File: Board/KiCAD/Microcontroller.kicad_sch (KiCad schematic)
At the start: 29 parts, among them J2 Conn_ARM_SWD_TagConnect_TC2030, J4 Conn_01x03, SW2 SW_Push, U5 LMR50410, U9 STM32F103C8T6, Y1 Crystal_GND24_Small, Y4 CM8V-T1A-32.768KHZ-12.5PF-20P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

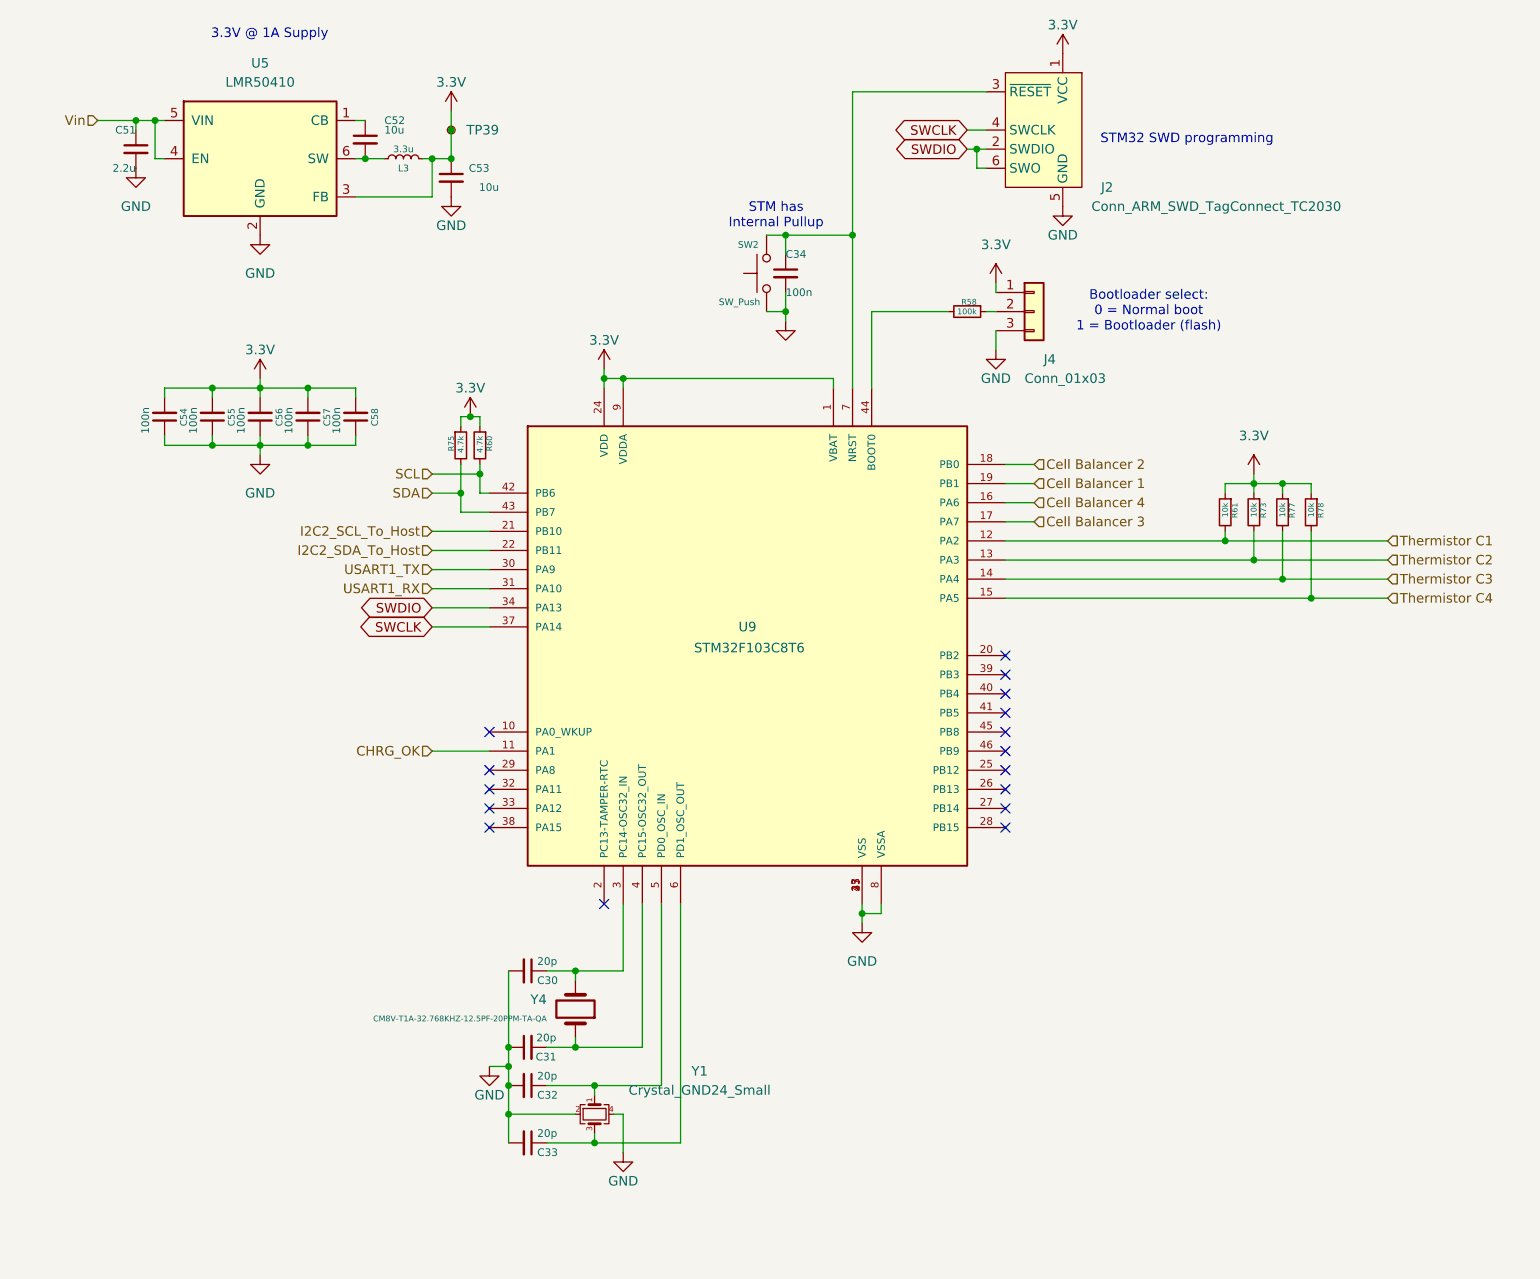
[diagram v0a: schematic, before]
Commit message: BOM Complete Need a Once Over Check
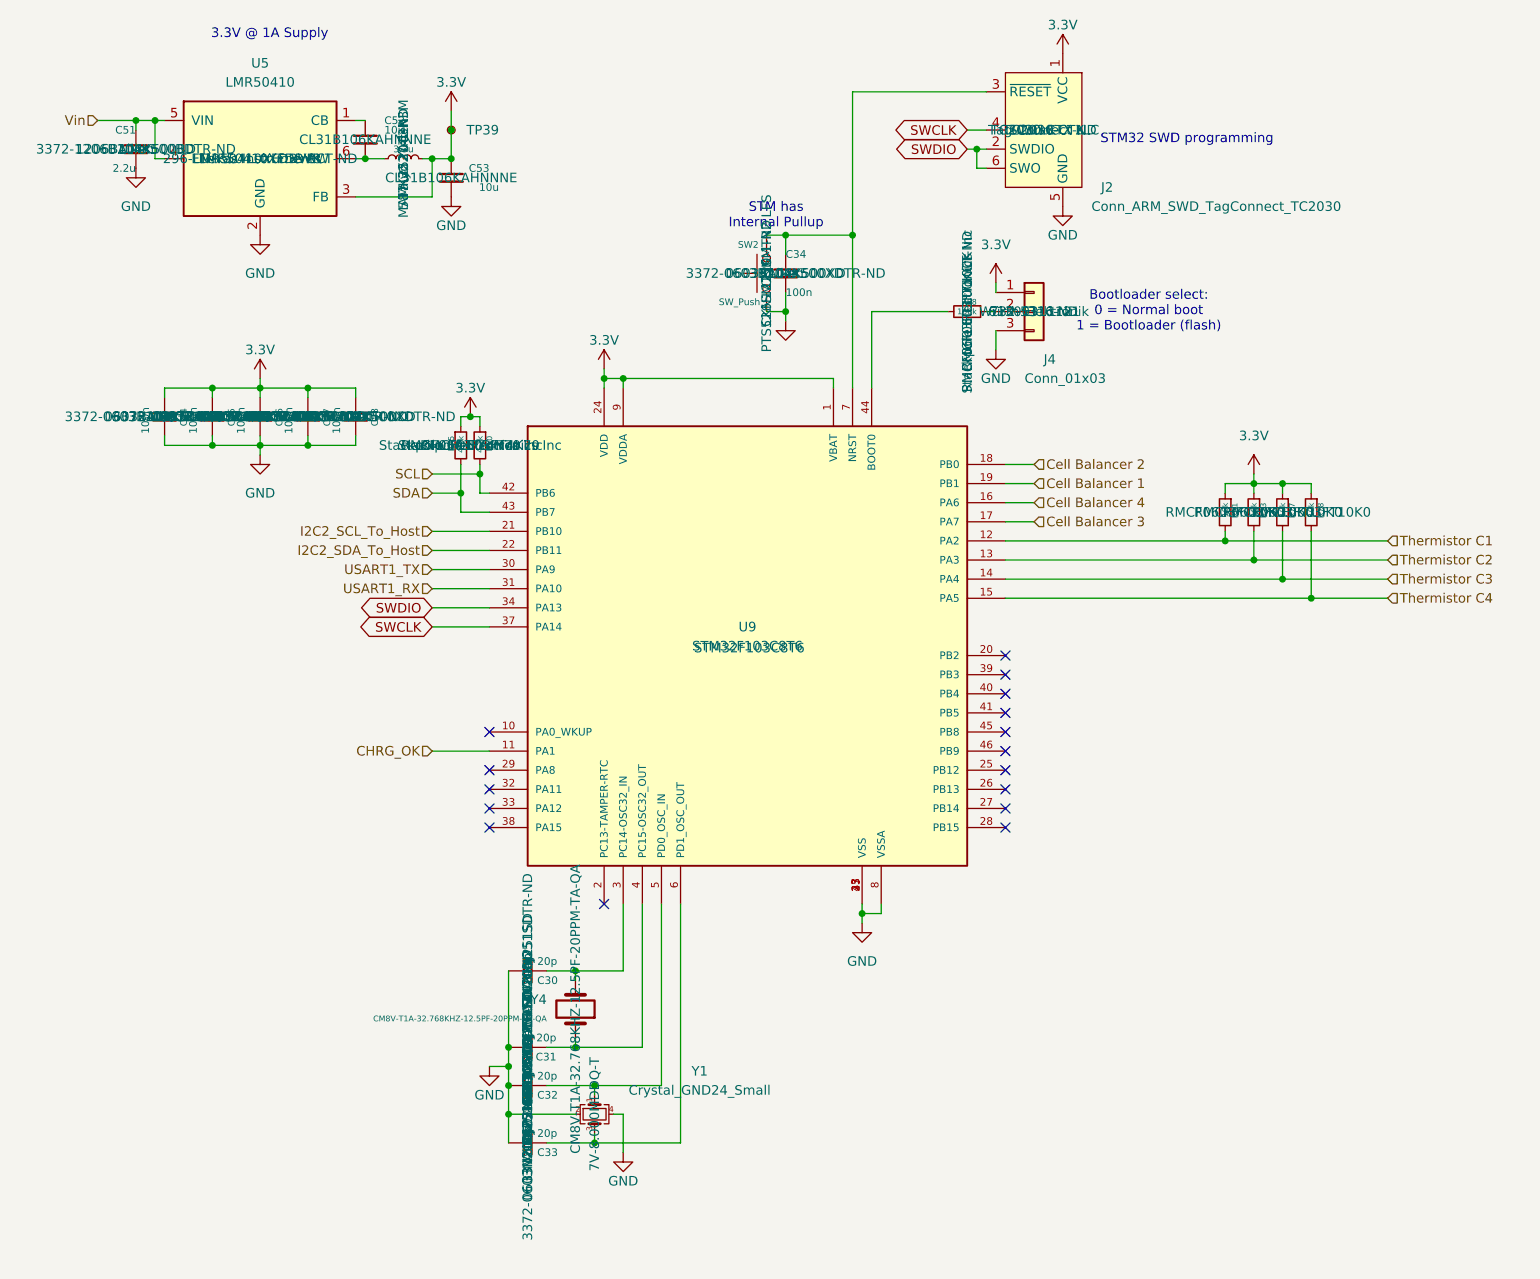
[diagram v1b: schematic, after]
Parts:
- C30, C31, C32, C33: MFR (none) -> Aillen; MPN (none) -> 3372-0603N200J251SDTR-ND; Package (none) -> 0603N200J251SD
- C34, C54, C55, C56, C57, C58: MFR (none) -> Aillen; MPN (none) -> 3372-0603B104K500XDTR-ND; Package (none) -> 0603B104K500XD
- C51: MFR (none) -> Aillen; MPN (none) -> 3372-1206B104K500BDTR-ND; Package (none) -> 1206B104K500BD
- C52, C53: MFR SAMSUNG -> Samsung Electro-Mechanics; MPN CL31A106KBHNNNE -> 1276-1804-1-ND; Package (none) -> CL31B106KAHNNNE
- J2: MFR (none) -> Tag-Connect LLC; MPN (none) -> TC2030-CTX-ND; Package (none) -> TC2030-CTX
- J4: MFR (none) -> Würth Elektronik; MPN (none) -> 732-5316-ND; Package (none) -> 61300311121
- L3: MFR (none) -> Taiyo Yuden; MPN (none) -> 587-3227-1-ND; Package (none) -> MAMK2520T3R3M
- R58: MFR (none) -> Stackpole Electronics Inc; MPN (none) -> RMCF0603FT100KCT-ND; Package (none) -> RMCF0603FT100K
- R60, R75: MFR (none) -> Stackpole Electronics Inc; MPN RMCF0603FT4K70 -> RMCF0603FT4K70CT-ND; Package (none) -> RMCF0603FT4K70
- R61, R73, R77, R78: MPN RMCF0603FT10K0 -> RMCF0603FT10K0CT-ND; Package (none) -> RMCF0603FT10K0
- SW2: MFR (none) -> C&K; MPN (none) -> CKN12220-1-ND; Package (none) -> PTS526SM15SMTR2 LFS
- U5: MFR (none) -> Texas Instruments; MPN (none) -> 296-LMR50410XFDBVRCT-ND; Package (none) -> LMR50410XFDBVR
- U9: Package (none) -> STM32F103C8T6
- Y1: Package (none) -> 7V-8.000MDDQ-T
- Y4: Package (none) -> CM8V-T1A-32.768KHZ-12.5PF-20PPM-TA-QA

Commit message: Updated schematic
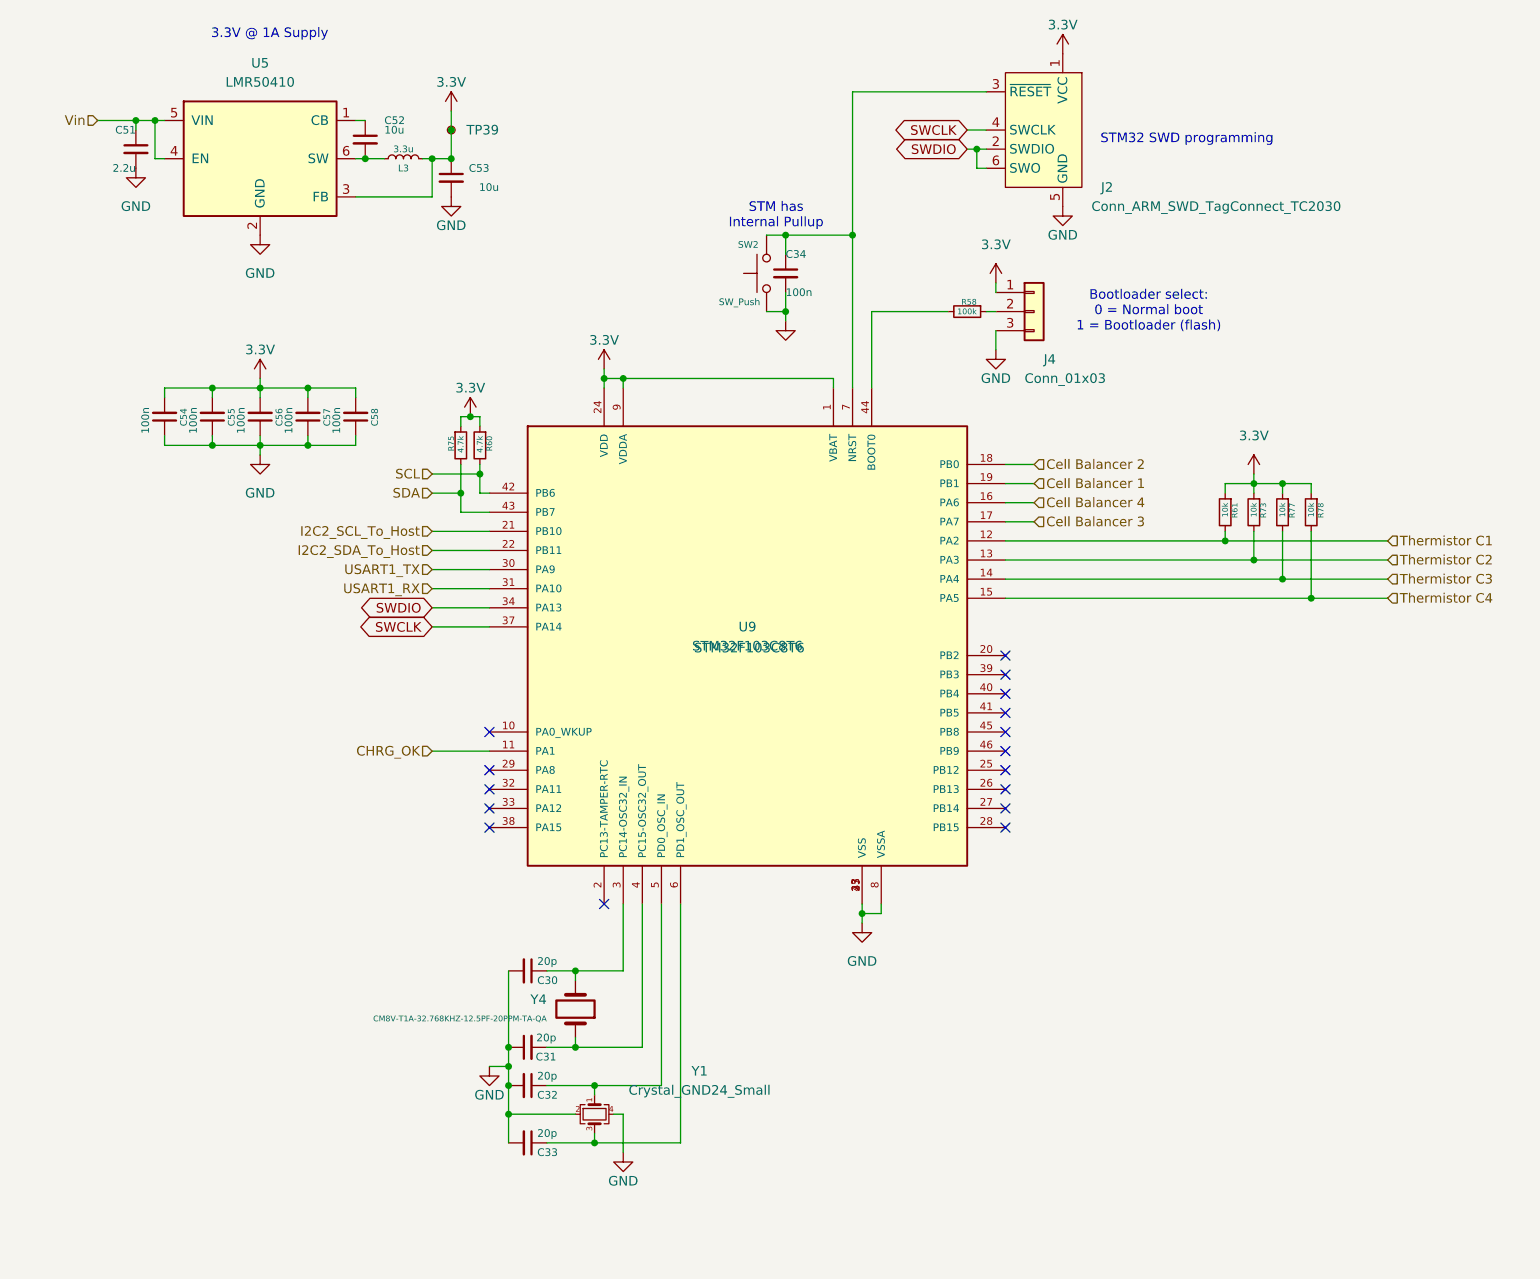
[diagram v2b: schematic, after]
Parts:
- R58: Package RMCF0603FT100K -> MCF0603FT100K
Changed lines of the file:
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@@
 					(size 1.27 1.27)
 				)
+				(hide yes)
 			)
 		)
@@
 					(size 1.27 1.27)
 				)
+				(hide yes)
 			)
 		)
@@
 					(size 1.27 1.27)
 				)
+				(hide yes)
 			)
 		)
@@
 					(size 1.27 1.27)
 				)
+				(hide yes)
 			)
 		)
@@
 					(size 1.27 1.27)
 				)
+				(hide yes)
 			)
 		)
@@
 					(size 1.27 1.27)
 				)
+				(hide yes)
 			)
 		)
@@
 					(size 1.27 1.27)
 				)
+				(hide yes)
 			)
 		)
@@
 					(size 1.27 1.27)
 				)
+				(hide yes)
 			)
 		)
@@
 					(size 1.27 1.27)
 				)
+				(hide yes)
 			)
 		)
@@
 					(size 1.27 1.27)
 				)
+				(hide yes)
 			)
 		)
@@
 					(size 1.27 1.27)
 				)
+				(hide yes)
 			)
 		)
@@
 					(size 1.27 1.27)
 				)
+				(hide yes)
 			)
 		)
@@
 					(size 1.27 1.27)
 				)
+				(hide yes)
 			)
 		)
@@
 					(size 1.27 1.27)
 				)
+				(hide yes)
 			)
 		)
@@
 					(size 1.27 1.27)
 				)
+				(hide yes)
 			)
 		)
@@
 					(size 1.27 1.27)
 				)
+				(hide yes)
 			)
 		)
@@
 					(size 1.27 1.27)
 				)
+				(hide yes)
 			)
 		)
@@
 					(size 1.27 1.27)
 				)
+				(hide yes)
 			)
 		)
@@
 					(size 1.27 1.27)
 				)
+				(hide yes)
 			)
 		)
@@
 					(size 1.27 1.27)
 				)
+				(hide yes)
 			)
 		)
@@
 					(size 1.27 1.27)
 				)
+				(hide yes)
 			)
 		)
@@
 			)
 		)
-		(property "Package" "RMCF0603FT100K"
+		(property "Package" "MCF0603FT100K"
 			(at 154.94 68.58 0)
 			(effects
@@
 					(size 1.27 1.27)
 				)
+				(hide yes)
 			)
 		)
@@
 					(size 1.27 1.27)
 				)
+				(hide yes)
 			)
 		)
@@
 					(size 1.27 1.27)
 				)
+				(hide yes)
 			)
 		)
@@
 					(size 1.27 1.27)
 				)
+				(hide yes)
 			)
 		)
@@
 					(size 1.27 1.27)
 				)
+				(hide yes)
 			)
 		)
@@
 					(size 1.27 1.27)
 				)
+				(hide yes)
 			)
 		)
@@
 					(size 1.27 1.27)
 				)
+				(hide yes)
 			)
 		)
@@
 					(size 1.27 1.27)
 				)
+				(hide yes)
 			)
 		)
@@
 					(size 1.27 1.27)
 				)
+				(hide yes)
 			)
 		)
@@
 					(size 1.27 1.27)
 				)
+				(hide yes)
 			)
 		)
@@
 					(size 1.27 1.27)
 				)
+				(hide yes)
 			)
 		)
@@
 					(size 1.27 1.27)
 				)
+				(hide yes)
 			)
 		)
@@
 					(size 1.27 1.27)
 				)
+				(hide yes)
 			)
 		)
@@
 					(size 1.27 1.27)
 				)
+				(hide yes)
 			)
 		)
@@
 					(size 1.27 1.27)
 				)
+				(hide yes)
 			)
 		)
@@
 					(size 1.27 1.27)
 				)
+				(hide yes)
 			)
 		)
@@
 					(size 1.27 1.27)
 				)
+				(hide yes)
 			)
 		)
@@
 					(size 1.27 1.27)
 				)
+				(hide yes)
 			)
 		)
@@
 					(size 1.27 1.27)
 				)
+				(hide yes)
 			)
 		)
@@
 					(size 1.27 1.27)
 				)
+				(hide yes)
 			)
 		)
@@
 					(size 1.27 1.27)
 				)
+				(hide yes)
 			)
 		)
@@
 					(size 1.27 1.27)
 				)
+				(hide yes)
 			)
 		)
@@
 					(size 1.27 1.27)
 				)
+				(hide yes)
 			)
 		)
@@
 					(size 1.27 1.27)
 				)
+				(hide yes)
 			)
 		)
@@
 					(size 1.27 1.27)
 				)
+				(hide yes)
 			)
 		)
@@
 					(size 1.27 1.27)
 				)
+				(hide yes)
 			)
 		)
@@
 					(size 1.27 1.27)
 				)
+				(hide yes)
 			)
 		)
@@
 					(size 1.27 1.27)
 				)
+				(hide yes)
 			)
 		)
@@
 					(size 1.27 1.27)
 				)
+				(hide yes)
 			)
 		)
@@
 					(size 1.27 1.27)
 				)
+				(hide yes)
 			)
 		)
@@
 					(size 1.27 1.27)
 				)
+				(hide yes)
 			)
 		)
@@
 					(size 1.27 1.27)
 				)
+				(hide yes)
 			)
 		)
@@
 					(size 1.27 1.27)
 				)
+				(hide yes)
 			)
 		)
@@
 					(size 1.27 1.27)
 				)
+				(hide yes)
 			)
 		)
@@
 					(size 1.27 1.27)
 				)
+				(hide yes)
 			)
 		)
@@
 					(size 1.27 1.27)
 				)
+				(hide yes)
 			)
 		)
@@
 					(size 1.27 1.27)
 				)
+				(hide yes)
 			)
 		)
@@
 					(size 1.27 1.27)
 				)
+				(hide yes)
 			)
 		)
@@
 					(size 1.27 1.27)
 				)
+				(hide yes)
 			)
 		)
@@
 					(size 1.27 1.27)
 				)
+				(hide yes)
 			)
 		)
@@
 					(size 1.27 1.27)
 				)
+				(hide yes)
 			)
 		)
@@
 					(size 1.27 1.27)
 				)
+				(hide yes)
 			)
 		)
